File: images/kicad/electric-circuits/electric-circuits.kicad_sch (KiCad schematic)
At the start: 66 parts, among them M1 motor

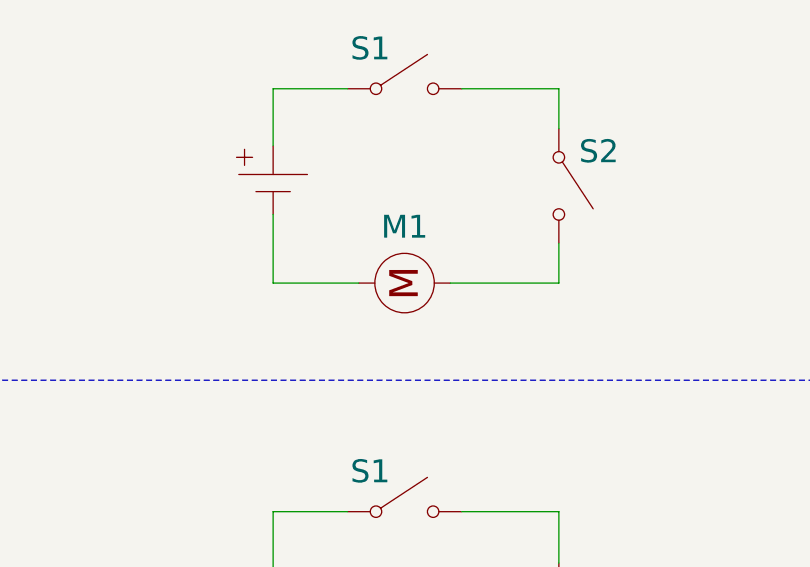
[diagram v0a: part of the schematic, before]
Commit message: 22/01/2025 Update
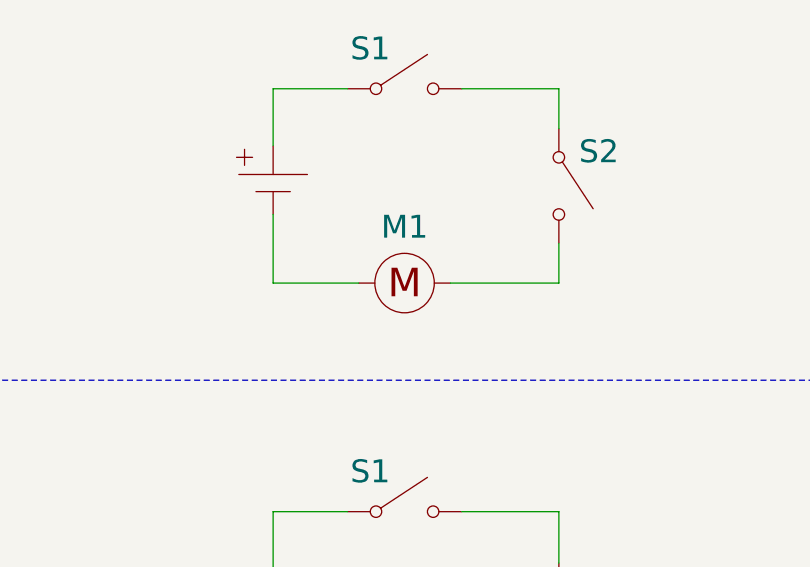
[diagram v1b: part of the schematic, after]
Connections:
- net at S?.: now also R?.; no longer V?.
- net at R?.: now also D?.; no longer S?.
- net at V?.: now also S?.; no longer R?.
- net at S?.: now also D?.; no longer V?.
- net at V?.: now also D3.; no longer R?. (x2)
- net at D3.: now also D1., D2.; no longer V?.
- net at D3.: now also D2.; no longer V?.
- net at V?.: now also S1., S2.; no longer Z?.
- net at S1., S2.: now also Z?.; no longer V?.
- net at V?.: now also L1., L3.; no longer S1.
- net at V?.: now also R?., S1.; no longer S2.
- net at R?., S1.: now also S2.; no longer V?.
- net at S1., S2.: now also R1.; no longer V?.
- net at V?.: now also M1.; no longer S1.
- net at M1.: now also S2.; no longer V?.
- net at V?.: now also S2.; no longer S1.
- net at S2.: now also R1.; no longer V?.
- net at V?.: now also L2.; no longer S1.
- net at L2.: now also L1.; no longer V?.
- net at V?.: now also L1., L2., S3.; no longer S1.
- net at V?.: now also L1., L2., S3., S4.; no longer S1.
- new net: S?., V?.
- new net: R?., V?. (x3)
- new net: V?., Z?.
- new net: S1., V?. (x6)
- new net: L2., S1., S2.
- new net: S2., V?.
- new net: S1., S2., V?.
- new net: R1., R2.
